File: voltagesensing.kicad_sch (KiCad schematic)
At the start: 10 parts, among them U3 AMC1200SDUBR

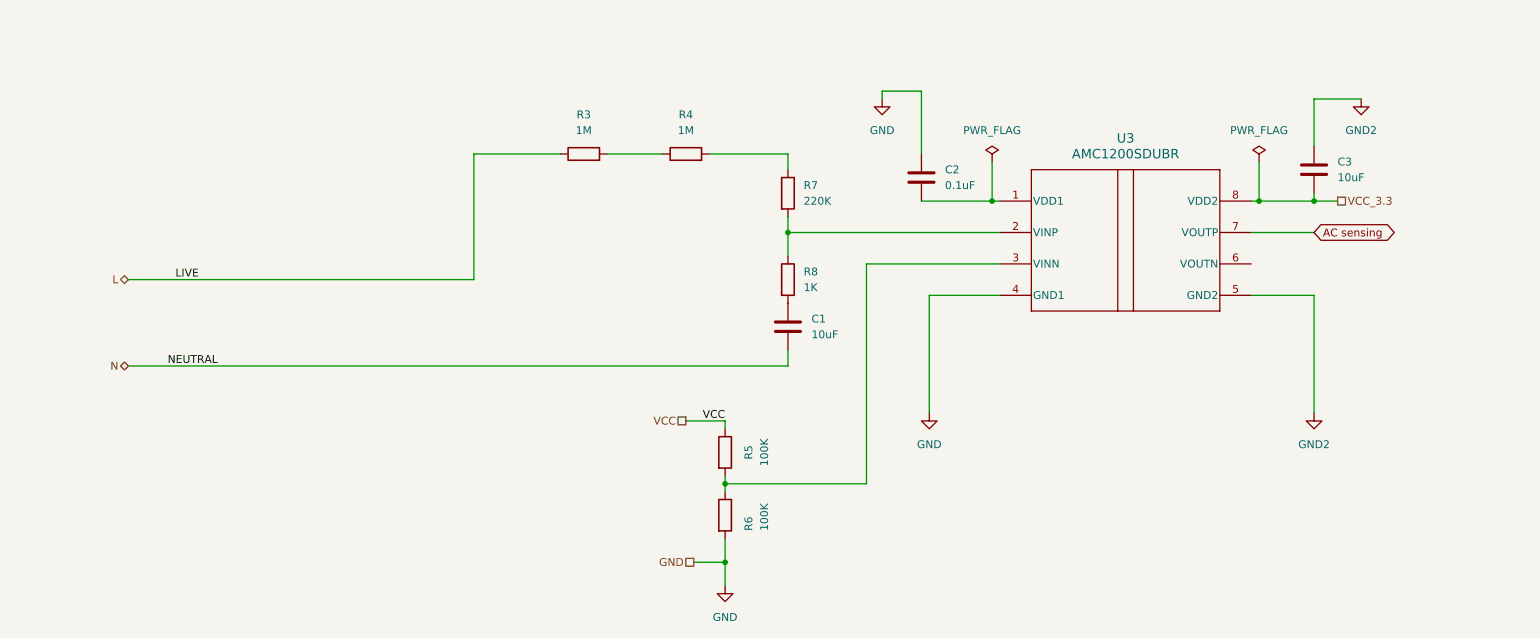
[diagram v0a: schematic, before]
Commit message: Final Schematic Editing Completed
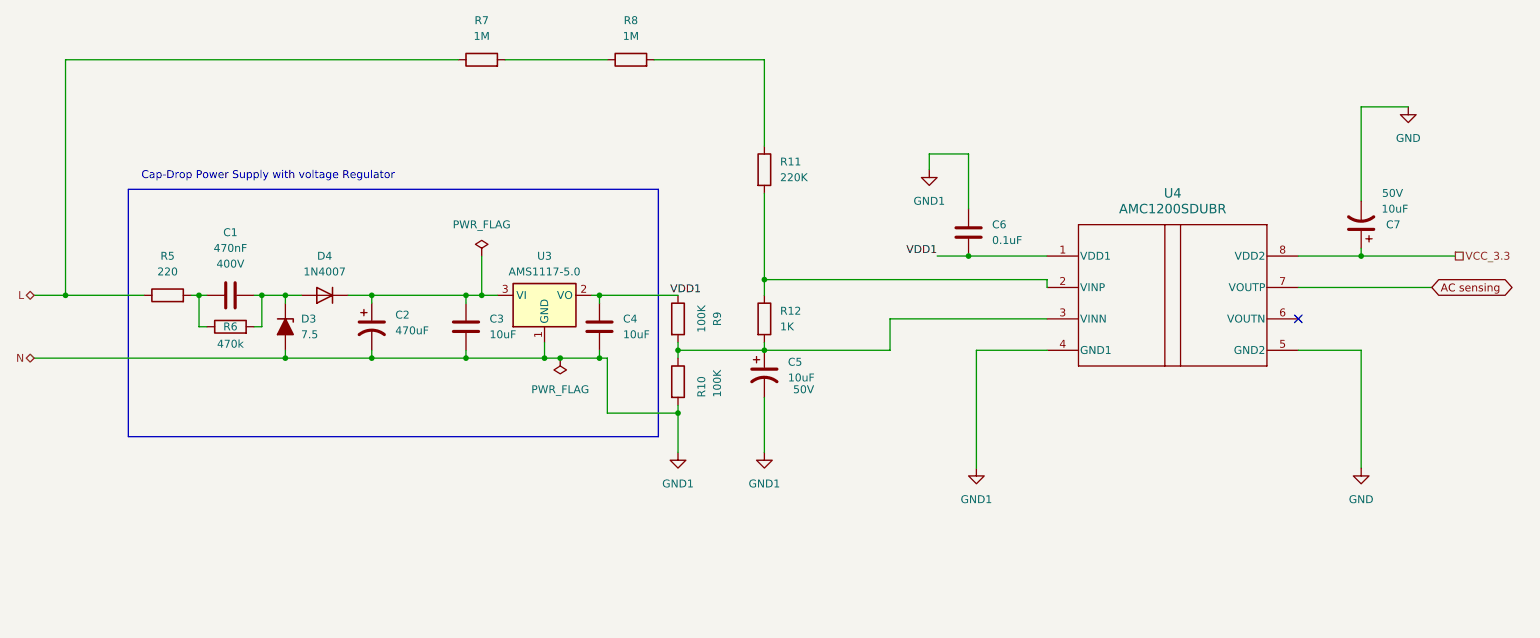
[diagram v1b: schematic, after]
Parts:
- removed R3, R4: 1M, Resistor_THT:R_Axial_DIN0207_L6.3mm_D2.5mm_P15.24mm_Horizontal, symbol Device:R
- removed U3: AMC1200SDUBR, DUB0008A-IPC_A, symbol 2025-08-05_00-17-59:AMC1200SDUBR
- added C2: 470uF, Capacitor_SMD:CP_Elec_6.3x7.7, symbol Device:C_Polarized_US
- added C4: 10uF, Capacitor_SMD:C_0402_1005Metric, symbol Device:C
- added C5, C7: 10uF, symbol Device:C_Polarized_US
- added D3: 7.5, Diode_SMD:D_MiniMELF, symbol Device:D_Zener_Filled
- added D4: 1N4007, Diode_THT:D_DO-41_SOD81_P10.16mm_Horizontal, symbol Diode:1N4007
- added R10, R9: 100K, Resistor_THT:R_Axial_DIN0207_L6.3mm_D2.5mm_P15.24mm_Horizontal, symbol Device:R
- added R11: 220K, Resistor_THT:R_Axial_DIN0207_L6.3mm_D2.5mm_P15.24mm_Horizontal, symbol Device:R
- added R12: 1K, Resistor_THT:R_Axial_DIN0207_L6.3mm_D2.5mm_P15.24mm_Horizontal, symbol Device:R
- added U3: AMS1117-5.0, Package_TO_SOT_SMD:SOT-223-3_TabPin2, symbol Regulator_Linear:AMS1117-5.0
- added U4: AMC1200SDUBR, DUB0008A-IPC_A, symbol 2025-08-05_00-17-59:AMC1200SDUBR
- C1: value 10uF -> 470nF; footprint Capacitor_SMD:C_0402_1005Metric -> Capacitor_THT:C_Rect_L32.0mm_W15.0mm_P27.00mm; voltage (none) -> 400V
- C3: footprint Capacitor_SMD:C_1206_3216Metric -> Capacitor_SMD:C_0402_1005Metric
- R5: value 100K -> 220; footprint Resistor_THT:R_Axial_DIN0207_L6.3mm_D2.5mm_P15.24mm_Horizontal -> Resistor_THT:R_Axial_DIN0414_L11.9mm_D4.5mm_P15.24mm_Horizontal
- R6: value 100K -> 470k
- R7: value 220K -> 1M
- R8: value 1K -> 1M
- renumbered C2 to C6
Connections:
- net VCC is gone; now on net L: R5.1
- net AC sensing: now also U4.7 (VOUTP)
- net GND: now also C7.2, U4.5 (GND2); no longer C6.1, R6.2
- net L: now also R7.1
- net VCC_3.3: now also C7.1, U4.8 (VDD2); no longer C3.2
- net at C1.1: now also R5.2, R6.1; no longer R8.2
- net VDD1: now reaches C6.2
- net VDD1: now also C4.1, R9.1, U3.2 (VO), U4.1 (VDD1)
- net GND2: no longer names the net of C3.1
- net GND2: now also C2.1, D4.1 (K), U3.3 (VI)
- net N: no longer names the net of C1.2
- net N: now also R6.2, D3.1 (K), D4.2 (A)
- new net: C5.1, R10.1, R12.2, R9.2, U4.3 (VINN)
- new net: R11.2, R12.1, U4.2 (VINP)
- new net: R11.1, R8.2
- new net GND1: C2.2, C3.2, C4.2, C5.2, C6.1, D3.2 (A), R10.2, U3.1 (GND), U4.4 (GND1)
- no-connect marks 0 -> 1
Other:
- note added: "Cap-Drop Power Supply with voltage Regulator"
- moved on the sheet: C6
